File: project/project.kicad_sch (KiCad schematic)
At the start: 65 parts, among them J1 Conn_02x16_Odd_Even, J2 TYPE-C 6P(040新), J3 Conn_01x02_Pin, SW1 SS-12D10L9, U1 DRV8833PWPR, U10 TPS22965DSGR, U2 CH224K, U3 DRV8833PWPR, U4 AP63203WU-7, U5 TP4056, U6 AP2114, U7 MT3608L, U8 INA219AIDCNR, U9 TPS22965DSGR

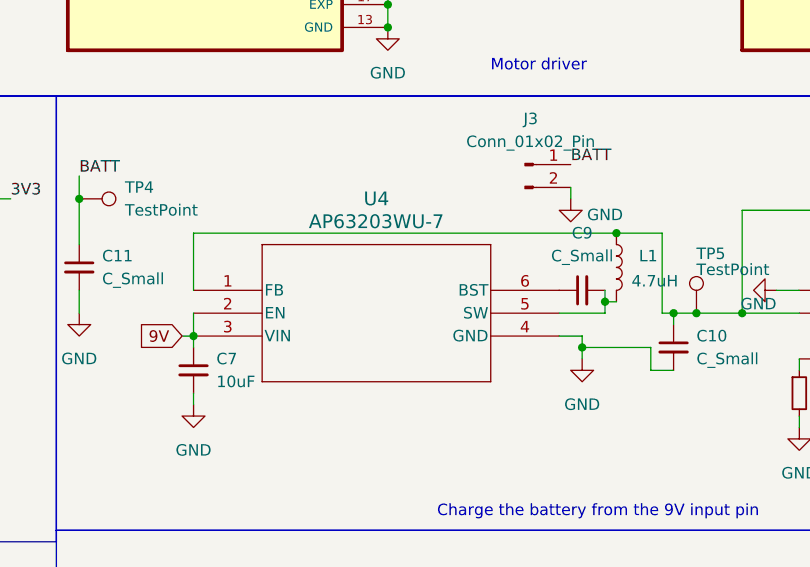
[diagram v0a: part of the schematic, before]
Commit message: update
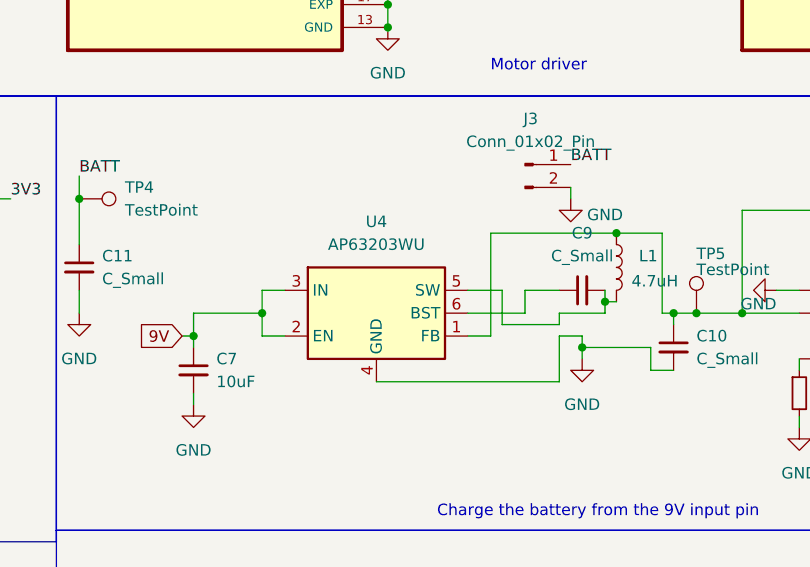
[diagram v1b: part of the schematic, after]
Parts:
- removed U4: AP63203WU-7, AP63203WU-7_DIO, symbol AP63203WU-7:AP63203WU-7
- added U4: AP63203WU, Package_TO_SOT_SMD:TSOT-23-6, symbol Regulator_Switching:AP63203WU
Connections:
- net 9V: now also U4.2 (EN), U4.3 (IN)
- net GND: now also U4.4 (GND)
- net at C10.1, D1.2 (A), D2.2 (A)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: now also U4.1 (FB)
- net at C9.2, L1.1: now also U4.5 (SW)
- net at C9.1: now also U4.6 (BST)
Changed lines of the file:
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@@
 	)
 	(junction
-		(at 143.51 92.71)
-		(diameter 0)
-		(color 0 0 0 0)
-	)
-	(junction
 		(at 68.58 88.9)
 		(diameter 0)
@@
 	)
 	(junction
+		(at 143.51 92.71)
+		(diameter 0)
+		(color 0 0 0 0)
+	)
+	(junction
 		(at 283.21 31.75)
 		(diameter 0)
@@
 	)
 	(junction
+		(at 104.14 101.6)
+		(diameter 0)
+		(color 0 0 0 0)
+	)
+	(junction
 		(at 149.86 101.6)
 		(diameter 0)
@@
 	(wire
 		(pts
+			(xy 130.81 99.06) (xy 130.81 102.87)
+		)
+		(stroke
+			(width 0)
+			(type default)
+		)
+	)
+	(wire
+		(pts
 			(xy 66.04 96.52) (xy 66.04 118.11)
 		)
@@
 	(wire
 		(pts
+			(xy 127 99.06) (xy 130.81 99.06)
+		)
+		(stroke
+			(width 0)
+			(type default)
+		)
+	)
+	(wire
+		(pts
 			(xy 251.46 31.75) (xy 261.62 31.75)
 		)
@@
 	(wire
 		(pts
+			(xy 137.16 109.22) (xy 116.84 109.22)
+		)
+		(stroke
+			(width 0)
+			(type default)
+		)
+	)
+	(wire
+		(pts
 			(xy 97.79 135.89) (xy 97.79 147.32)
 		)
@@
 	(wire
 		(pts
+			(xy 133.35 99.06) (xy 137.16 99.06)
+		)
+		(stroke
+			(width 0)
+			(type default)
+		)
+	)
+	(wire
+		(pts
 			(xy 100.33 147.32) (xy 100.33 148.59)
 		)
@@
 	(wire
 		(pts
-			(xy 96.52 92.71) (xy 96.52 99.06)
+			(xy 96.52 101.6) (xy 104.14 101.6)
+		)
+		(stroke
+			(width 0)
+			(type default)
+		)
+	)
+	(wire
+		(pts
+			(xy 137.16 102.87) (xy 137.16 101.6)
 		)
 		(stroke
@@
 	(wire
 		(pts
+			(xy 129.54 104.14) (xy 129.54 92.71)
+		)
+		(stroke
+			(width 0)
+			(type default)
+		)
+	)
+	(wire
+		(pts
 			(xy 203.2 78.74) (xy 199.39 78.74)
 		)
@@
 	(wire
 		(pts
+			(xy 104.14 104.14) (xy 106.68 104.14)
+		)
+		(stroke
+			(width 0)
+			(type default)
+		)
+	)
+	(wire
+		(pts
 			(xy 163.83 149.86) (xy 163.83 151.13)
 		)
@@
 	(wire
 		(pts
+			(xy 137.16 104.14) (xy 137.16 109.22)
+		)
+		(stroke
+			(width 0)
+			(type default)
+		)
+	)
+	(wire
+		(pts
+			(xy 104.14 99.06) (xy 106.68 99.06)
+		)
+		(stroke
+			(width 0)
+			(type default)
+		)
+	)
+	(wire
+		(pts
 			(xy 194.31 104.14) (xy 203.2 104.14)
 		)
@@
 	(wire
 		(pts
+			(xy 130.81 102.87) (xy 137.16 102.87)
+		)
+		(stroke
+			(width 0)
+			(type default)
+		)
+	)
+	(wire
+		(pts
 			(xy 134.62 24.13) (xy 152.4 24.13)
 		)
@@
 	(wire
 		(pts
+			(xy 104.14 101.6) (xy 104.14 99.06)
+		)
+		(stroke
+			(width 0)
+			(type default)
+		)
+	)
+	(wire
+		(pts
 			(xy 66.04 118.11) (xy 26.67 118.11)
 		)
@@
 	(wire
 		(pts
+			(xy 127 101.6) (xy 133.35 101.6)
+		)
+		(stroke
+			(width 0)
+			(type default)
+		)
+	)
+	(wire
+		(pts
 			(xy 276.86 36.83) (xy 279.4 36.83)
 		)
@@
 	(wire
 		(pts
+			(xy 104.14 101.6) (xy 104.14 104.14)
+		)
+		(stroke
+			(width 0)
+			(type default)
+		)
+	)
+	(wire
+		(pts
 			(xy 151.13 31.75) (xy 152.4 31.75)
 		)
@@
 	(wire
 		(pts
+			(xy 129.54 92.71) (xy 143.51 92.71)
+		)
+		(stroke
+			(width 0)
+			(type default)
+		)
+	)
+	(wire
+		(pts
 			(xy 95.25 104.14) (xy 96.52 104.14)
 		)
@@
 	(wire
 		(pts
-			(xy 354.33 27.94) (xy 359.41 27.94)
+			(xy 127 104.14) (xy 129.54 104.14)
 		)
 		(stroke
@@
 	(wire
 		(pts
-			(xy 96.52 92.71) (xy 143.51 92.71)
+			(xy 354.33 27.94) (xy 359.41 27.94)
 		)
 		(stroke
@@
 	(wire
 		(pts
+			(xy 133.35 101.6) (xy 133.35 99.06)
+		)
+		(stroke
+			(width 0)
+			(type default)
+		)
+	)
+	(wire
+		(pts
 			(xy 161.29 143.51) (xy 163.83 143.51)
 		)
@@
 	)
 	(symbol
-		(lib_id "AP63203WU-7:AP63203WU-7")
-		(at 96.52 99.06 0)
-		(unit 1)
-		(exclude_from_sim no)
-		(in_bom yes)
-		(on_board yes)
-		(dnp no)
-		(fields_autoplaced yes)
-		(property "Reference" "U4"
-			(at 116.84 88.9 0)
-			(effects
-				(font
-					(size 1.524 1.524)
-				)
-			)
-		)
-		(property "Value" "AP63203WU-7"
-			(at 116.84 91.44 0)
-			(effects
-				(font
-					(size 1.524 1.524)
-				)
-			)
-		)
-		(property "Footprint" "AP63203WU-7_DIO"
-			(at 96.52 99.06 0)
-			(effects
-				(font
-					(size 1.27 1.27)
-					(italic yes)
-				)
-				(hide yes)
-			)
-		)
-		(property "Datasheet" "AP63203WU-7"
-			(at 96.52 99.06 0)
-			(effects
-				(font
-					(size 1.27 1.27)
-					(italic yes)
-				)
-				(hide yes)
-			)
-		)
-		(property "Description" ""
-			(at 96.52 99.06 0)
-			(effects
-				(font
-					(size 1.27 1.27)
-				)
-				(hide yes)
-			)
-		)
-		(pin "1"
-		)
-		(pin "6"
-		)
-		(pin "3"
-		)
-		(pin "5"
-		)
-		(pin "4"
-		)
-		(pin "2"
-		)
-		(instances
-			(project "project"
-				(path "/f99403a2-5f0d-4f36-8249-ee7d0699b27a"
-					(reference "U4")
-					(unit 1)
-				)
-			)
-		)
-	)
-	(symbol
 		(lib_id "power:GND")
 		(at 118.11 69.85 0)
@@
 					(unit 1)
 				)
+			)
+		)
+	)
+	(symbol
+		(lib_id "Regulator_Switching:AP63203WU")
+		(at 116.84 101.6 0)
+		(unit 1)
+		(exclude_from_sim no)
+		(in_bom yes)
+		(on_board yes)
+		(dnp no)
+		(fields_autoplaced yes)
+		(property "Reference" "U4"
+			(at 116.84 91.44 0)
+			(effects
+				(font
+					(size 1.27 1.27)
+				)
+			)
+		)
+		(property "Value" "AP63203WU"
+			(at 116.84 93.98 0)
+			(effects
+				(font
+					(size 1.27 1.27)
+				)
+			)
+		)
+		(property "Footprint" "Package_TO_SOT_SMD:TSOT-23-6"
+			(at 116.84 124.46 0)
+			(effects
+				(font
+					(size 1.27 1.27)
+				)
+				(hide yes)
+			)
+		)
+		(property "Datasheet" "https://www.diodes.com/assets/Datasheets/AP63200-AP63201-AP63203-AP63205.pdf"
+			(at 116.84 101.6 0)
+			(effects
+				(font
+					(size 1.27 1.27)
+				)
+				(hide yes)
+			)
+		)
+		(property "Description" "2A, 1.1MHz Buck DC/DC Converter, fixed 3.3V output voltage, TSOT-23-6"
+			(at 116.84 101.6 0)
+			(effects
+				(font
+					(size 1.27 1.27)
+				)
+				(hide yes)
+			)
+		)
+		(pin "1"
+		)
+		(pin "3"
+		)
+		(pin "2"
+		)
+		(pin "4"
+		)
+		(pin "5"
+		)
+		(pin "6"
+		)
+		(instances
+			(project ""
+				(path "/f99403a2-5f0d-4f36-8249-ee7d0699b27a"
+					(reference "U4")
+					(unit 1)
+				)

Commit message: Footprints updated
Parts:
- U1, U3: footprint DRV8833PWPR:IC_DRV8833PWPR -> Footprint:DRV8833PWPR
- U10, U9: footprint TPS22965DSGR:SON50P200X200X80-9N -> Footprint:TPS22965DSGR
- U5: footprint TP4056:SOP127P600X175-9N -> Footprint:TP4056
- U8: footprint INA219AIDCNR:SOT65P280X145-8N -> Footprint:INA219AIDCNR
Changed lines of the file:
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@@
 			)
 		)
-		(property "Footprint" "TPS22965DSGR:SON50P200X200X80-9N"
+		(property "Footprint" "Footprint:TPS22965DSGR"
 			(at 119.38 147.32 0)
 			(effects
@@
 			)
 		)
-		(property "Footprint" "TP4056:SOP127P600X175-9N"
+		(property "Footprint" "Footprint:TP4056"
 			(at 179.07 104.14 0)
 			(effects
@@
 			)
 		)
-		(property "Footprint" "TPS22965DSGR:SON50P200X200X80-9N"
+		(property "Footprint" "Footprint:TPS22965DSGR"
 			(at 182.88 143.51 0)
 			(effects
@@
 			)
 		)
-		(property "Footprint" "DRV8833PWPR:IC_DRV8833PWPR"
+		(property "Footprint" "Footprint:DRV8833PWPR"
 			(at 172.72 46.99 0)
 			(effects
@@
 			)
 		)
-		(property "Footprint" "DRV8833PWPR:IC_DRV8833PWPR"
+		(property "Footprint" "Footprint:DRV8833PWPR"
 			(at 97.79 46.99 0)
 			(effects
@@
 			)
 		)
-		(property "Footprint" "INA219AIDCNR:SOT65P280X145-8N"
+		(property "Footprint" "Footprint:INA219AIDCNR"
 			(at 46.99 101.6 0)
 			(effects
